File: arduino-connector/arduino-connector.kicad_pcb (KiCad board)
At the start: 2 copper layers, 121 x 69 mm, 13 parts, among them J1 Controller Connection, SW1 5V Switch, SW2 3V3 Switch, SW3 DIR_B / DIR_C, SW4 STP_B / STP_C

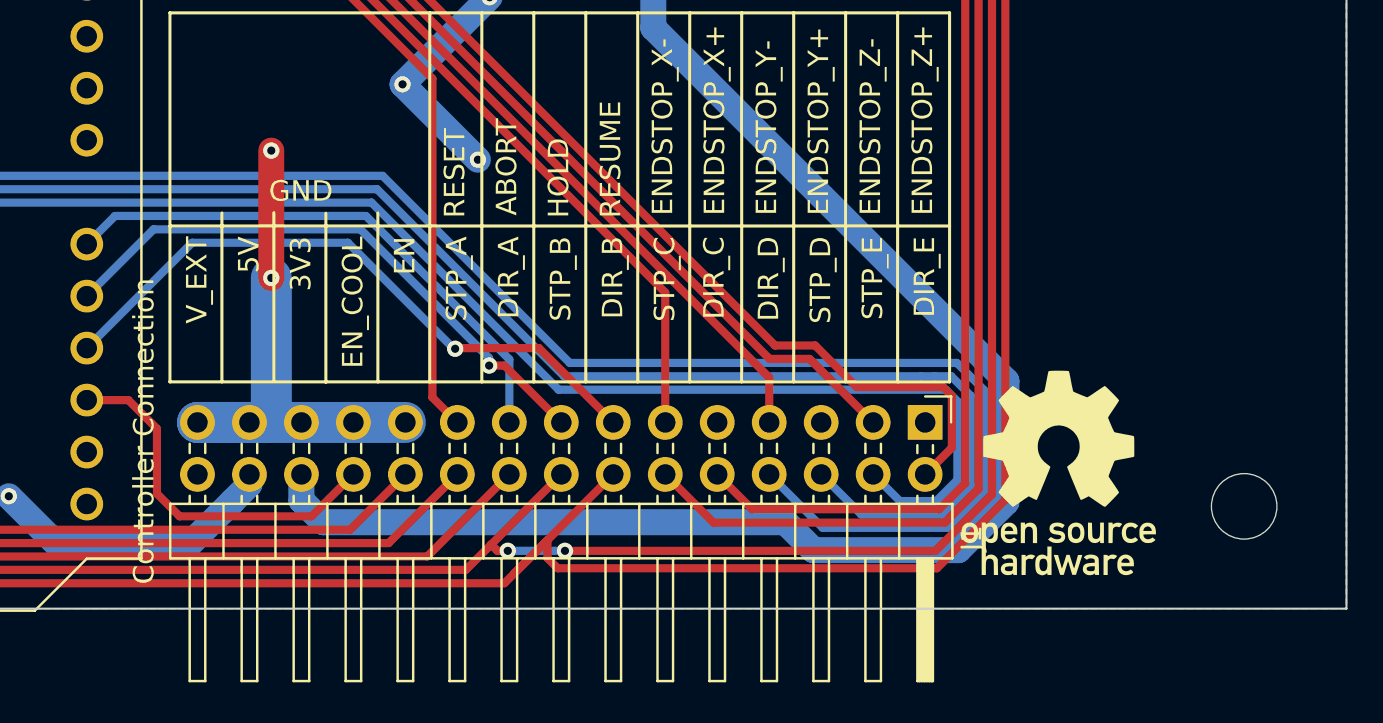
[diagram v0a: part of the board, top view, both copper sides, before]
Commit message: Added Gerber Files for each Circuit Board
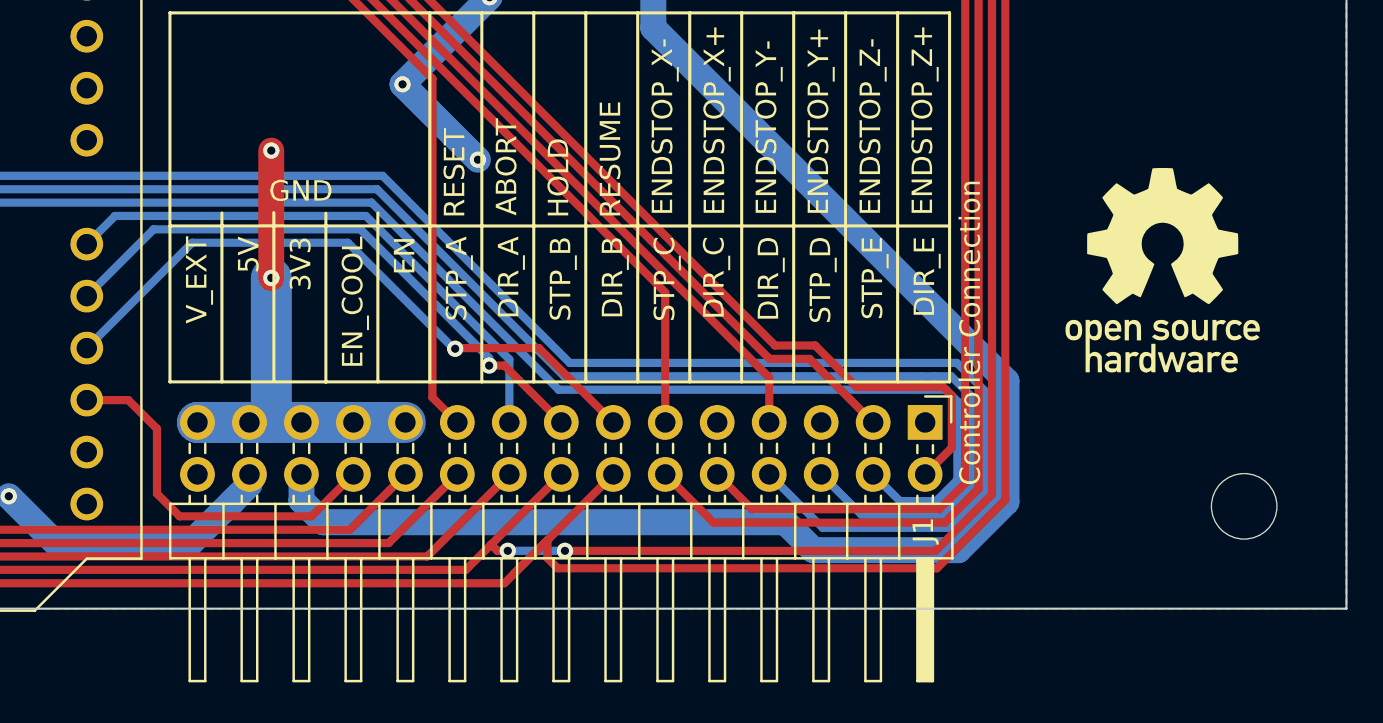
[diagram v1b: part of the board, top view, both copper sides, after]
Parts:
- moved G*** 11.1 mm to (144.0, 108.5)
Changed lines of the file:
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@@
       (drillshape 0)
       (scaleselection 1)
-      (outputdirectory "")
+      (outputdirectory "Gerber Files/V1.0.1/")
     )
   )
@@
     (property "ki_keywords" "connector")
     (attr through_hole)
-    (fp_text reference "J1" (at 5.655 -2.27 90) (layer "F.SilkS")
+    (fp_text reference "J1" (at 5.258 0.076 90) (layer "F.SilkS")
         (effects (font (size 1 1) (thickness 0.15)))
     )
-    (fp_text value "Controller Connection" (at 0.432 38.176 90) (layer "F.SilkS")
+    (fp_text value "Controller Connection" (at -4.394 -2.21 90) (layer "F.SilkS")
         (effects (font (size 1 1) (thickness 0.15)))
     )
@@
   )
   (footprint "logos:OHS Logo" (layer "F.Cu")
-    (at 138.938 118.364)
+    (at 144.018 108.458)
     (attr board_only exclude_from_pos_files exclude_from_bom)
     (fp_text reference "G***" (at 0 0) (layer "F.SilkS") hide
@@
     (connect_pads (clearance 0.5))
     (min_thickness 0.25) (filled_areas_thickness no)
-    (fill (thermal_gap 0.5) (thermal_bridge_width 0.5))
+    (fill yes (thermal_gap 0.5) (thermal_bridge_width 0.5))
     (polygon
       (pts
@@
     (connect_pads (clearance 0.5))
     (min_thickness 0.25) (filled_areas_thickness no)
-    (fill (thermal_gap 0.5) (thermal_bridge_width 0.5))
+    (fill yes (thermal_gap 0.5) (thermal_bridge_width 0.5))
     (polygon
       (pts
